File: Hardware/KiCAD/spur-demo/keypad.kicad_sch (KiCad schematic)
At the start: 40 parts, among them SW10 DOWN, SW11 7, SW12 8, SW13 9, SW14 LEFT, SW15 *, SW16 0, SW17 #, SW18 RIGHT, SW19 PTT, SW20 MENU, SW21 EXIT, SW22 SK0, SW3 1, SW4 2, SW5 3, SW6 UP, SW7 4, SW8 5, SW9 6

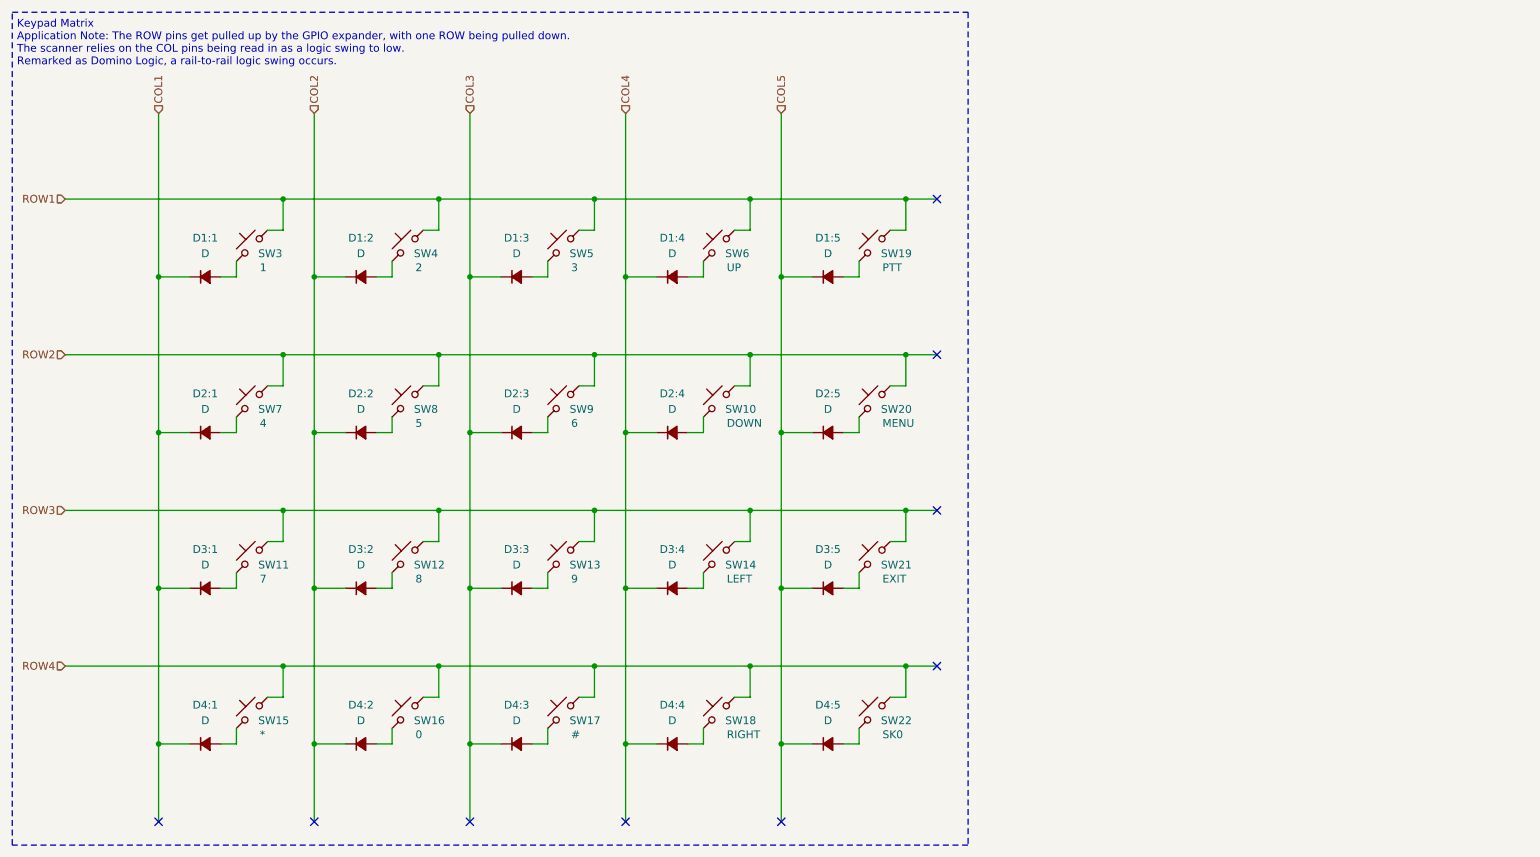
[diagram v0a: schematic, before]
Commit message: feat: squash recaptured schematics and footprint reassignments
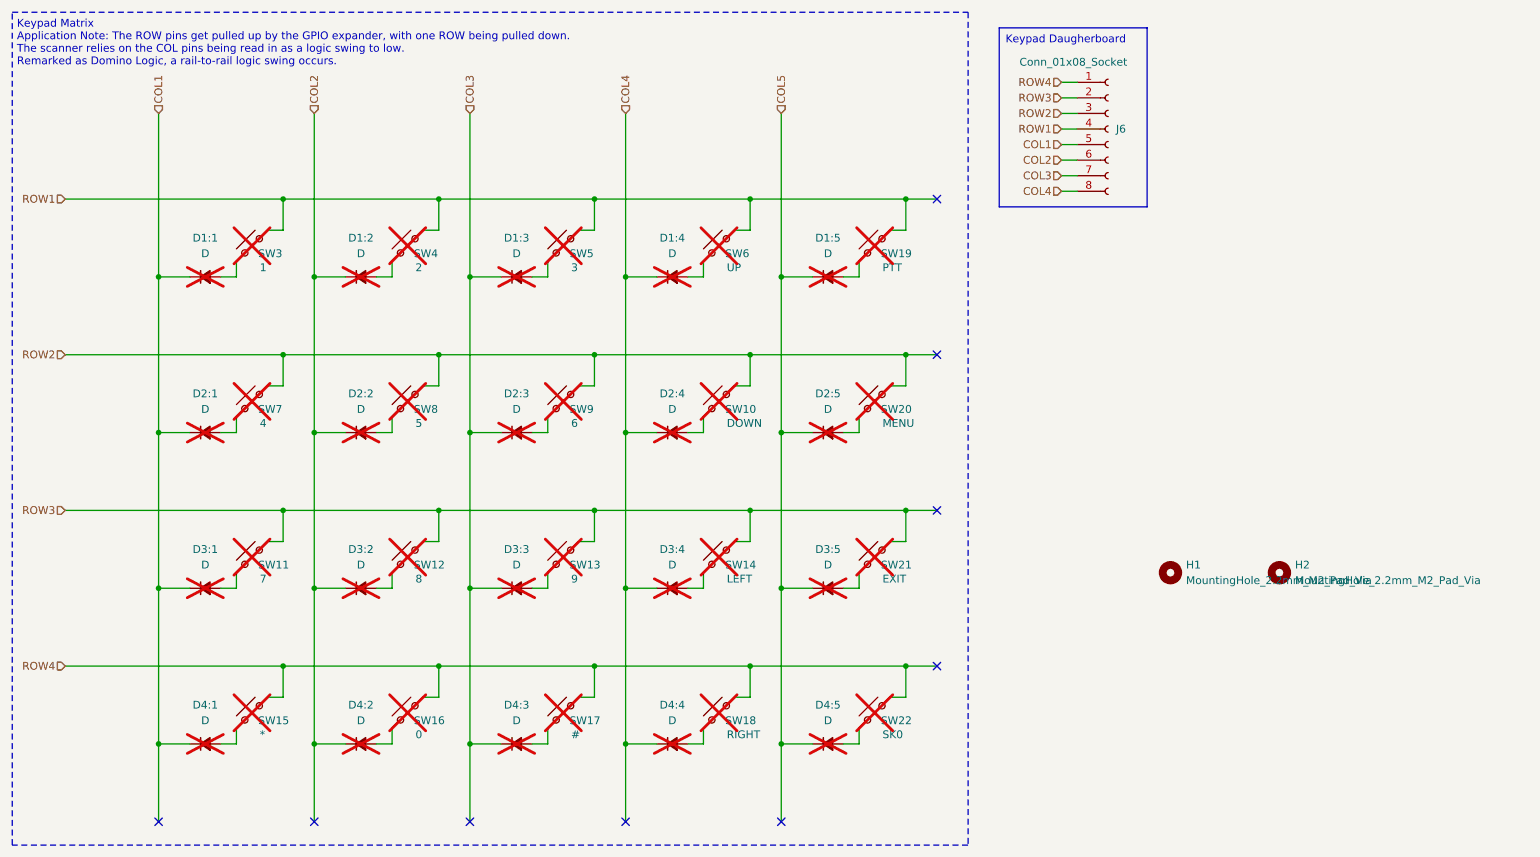
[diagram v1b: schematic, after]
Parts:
- added H1, H2: MountingHole_2.2mm_M2_Pad_Via, MountingHole:MountingHole_2.2mm_M2_Pad_Via, symbol Mechanical:MountingHole
- added J6: Conn_01x08_Socket, spur-demo:HW-834, symbol Connector:Conn_01x08_Socket
- D1:1, D1:2, D1:3, D1:4, D1:5, D2:1, D2:2, D2:3, D2:4, D2:5, D3:1, D3:2, D3:3, D3:4, D3:5, D4:1, D4:2, D4:3, D4:4, D4:5, SW10, SW11, SW12, SW13, SW14, SW15, SW16, SW17, SW18, SW19, SW20, SW21, SW22, SW3, SW4, SW5, SW6, SW7, SW8, SW9: now not fitted; now left out of the parts list
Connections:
- net COL1: now also J6.5 (Pin_5)
- net COL2: now also J6.6 (Pin_6)
- net COL3: now also J6.7 (Pin_7)
- net COL4: now also J6.8 (Pin_8)
- net ROW1: now also J6.4 (Pin_4)
- net ROW2: now also J6.3 (Pin_3)
- net ROW3: now also J6.2 (Pin_2)
- net ROW4: now also J6.1 (Pin_1)
